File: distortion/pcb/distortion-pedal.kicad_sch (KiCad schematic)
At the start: 22 parts, among them U2 TL081H, U4 TL081H

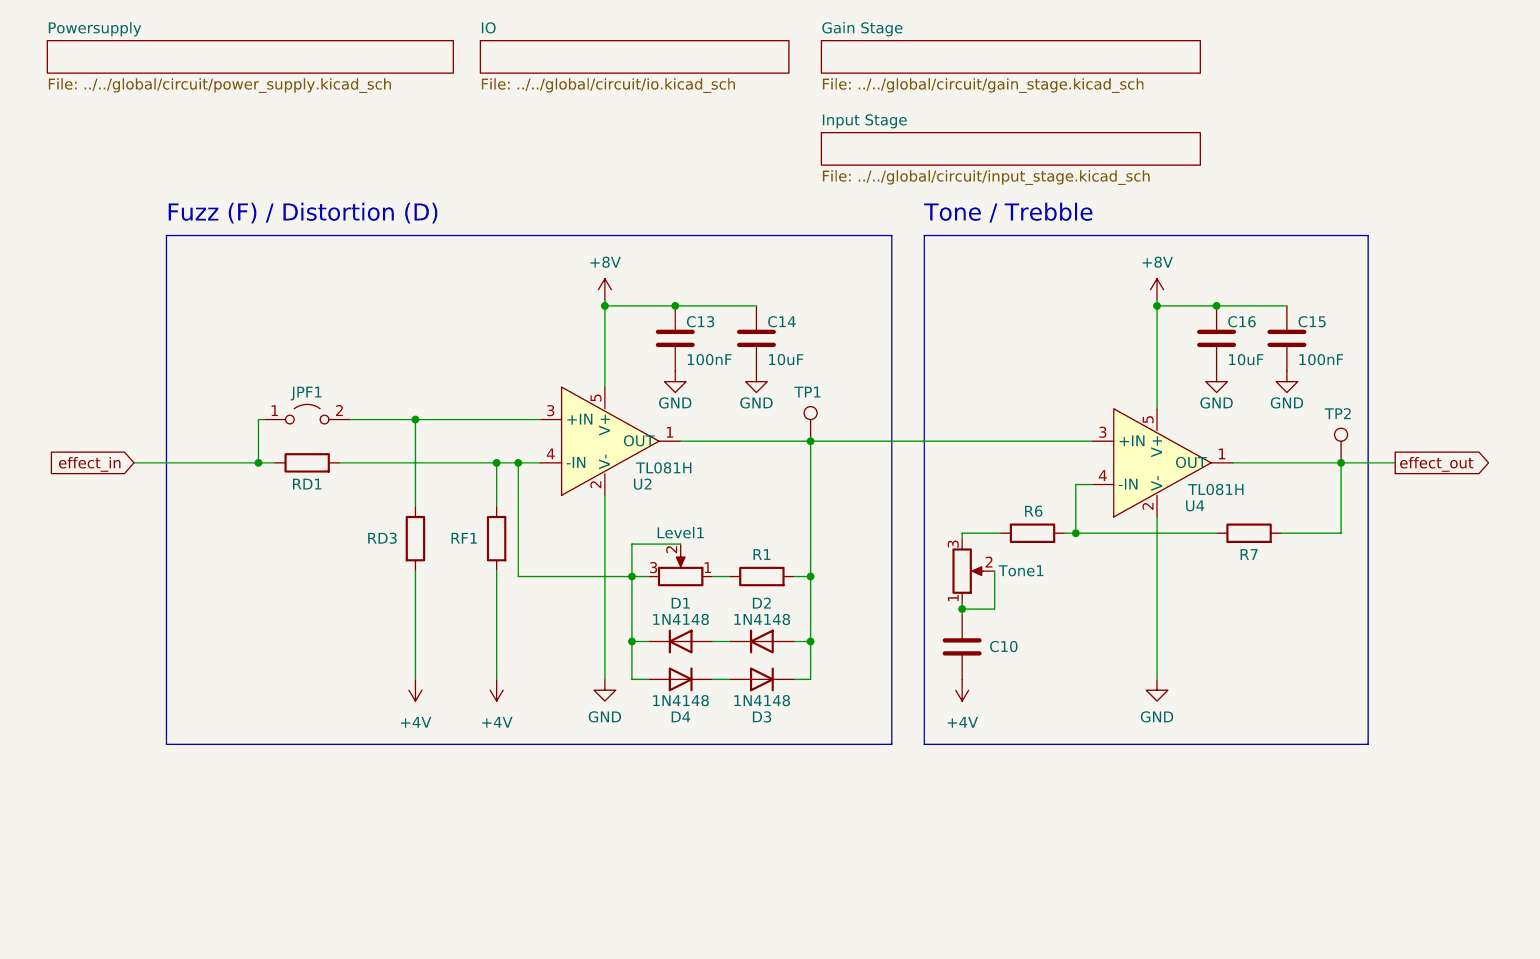
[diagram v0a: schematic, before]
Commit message: distortion rev 3
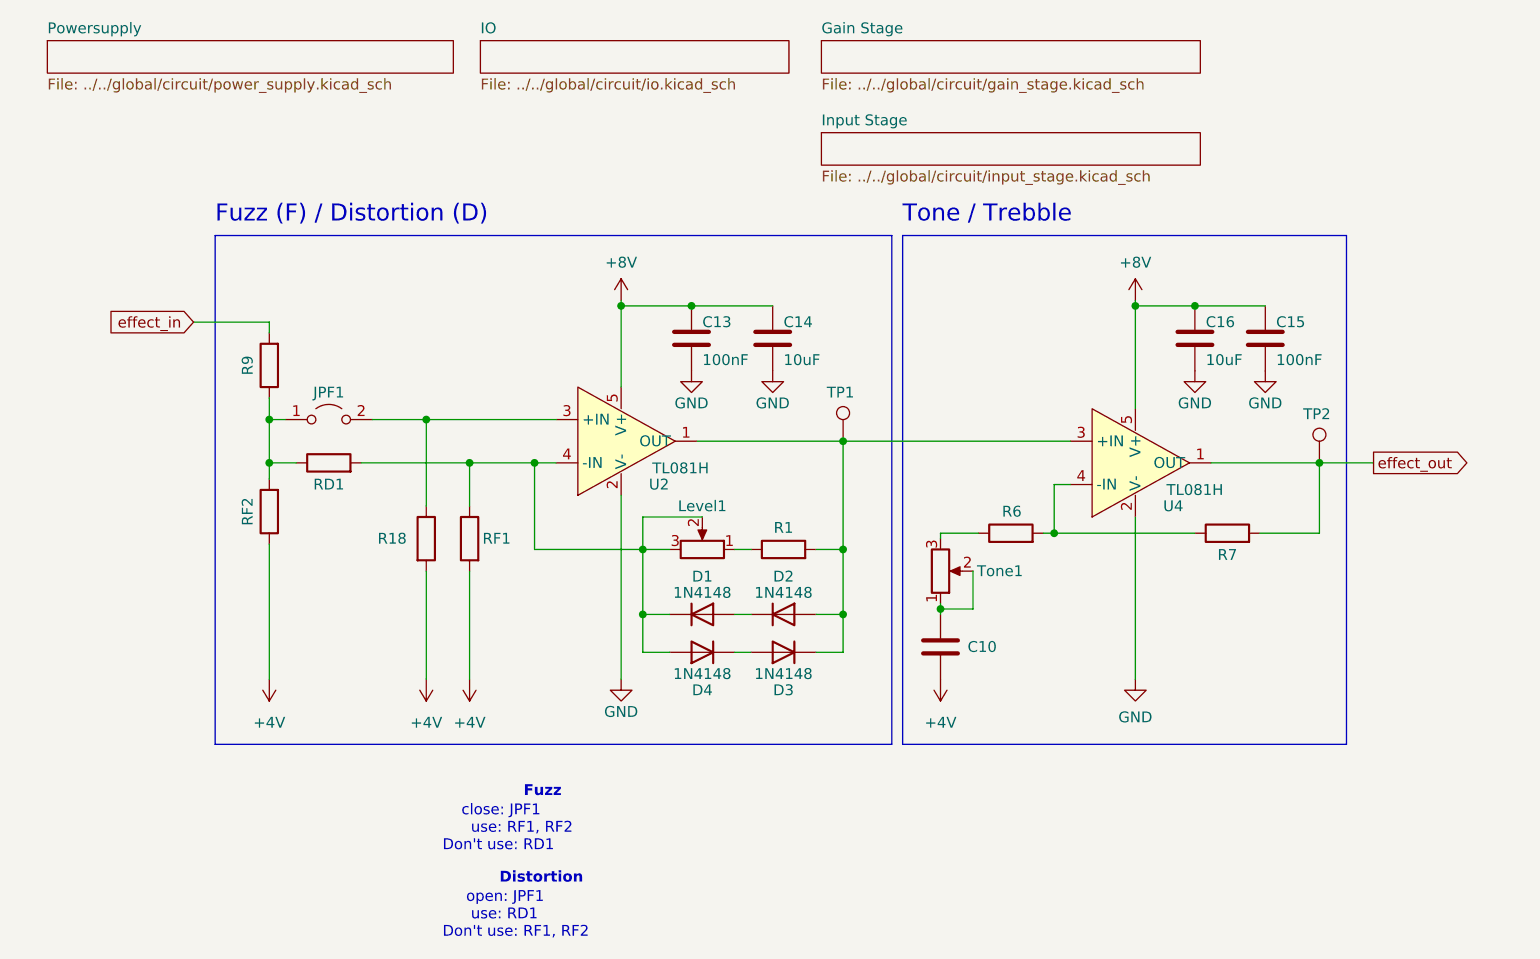
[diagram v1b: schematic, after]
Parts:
- added R9, RF2: R, Resistor_SMD:R_0805_2012Metric_Pad1.20x1.40mm_HandSolder, symbol Device:R
- Level1: footprint Connector_PinHeader_2.54mm:PinHeader_1x03_P2.54mm_Vertical -> effect_pedal:potentiometer_wired_23_connected
- Tone1: footprint Connector_PinHeader_2.54mm:PinHeader_1x03_P2.54mm_Vertical -> effect_pedal:potentiometer_wired_12_connected
- renumbered RD3 to R18
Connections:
- net +4V: now also RF2.1
- net effect_in: now also R9.2; no longer JPF1.1 (A), RD1.1
- new net: JPF1.1 (A), R9.1, RD1.1, RF2.2
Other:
- note added: "Distortion"
- note added: "Fuzz"
- note added: "close: JPF1 use: RF1, RF2 Don't use: RD1"
- note added: "open: JPF1 use: RD1 Don't use: RF1, RF2"
- moved on the sheet: C10, C13, C14, C15, C16, D1, D2, D3, D4, JPF1, Level1, R1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
